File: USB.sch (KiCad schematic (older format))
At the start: 47 parts

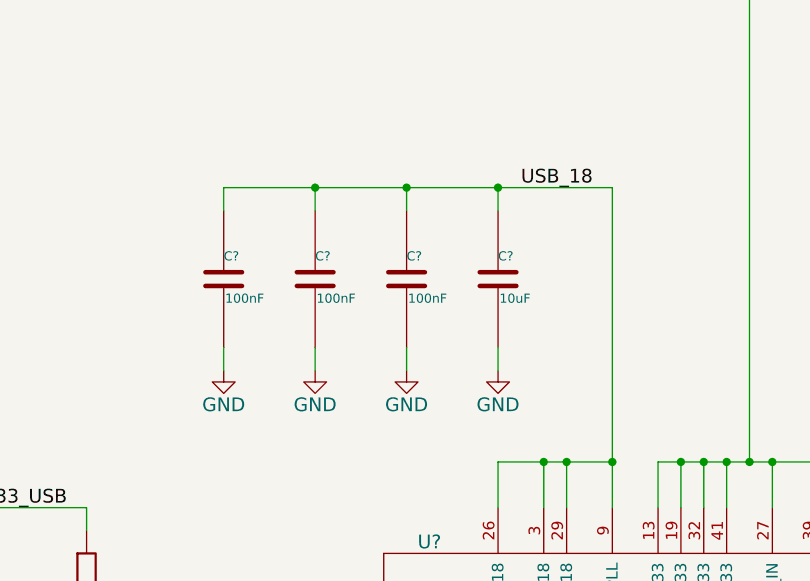
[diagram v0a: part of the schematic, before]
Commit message: moved a bunch of things around inside the schematics
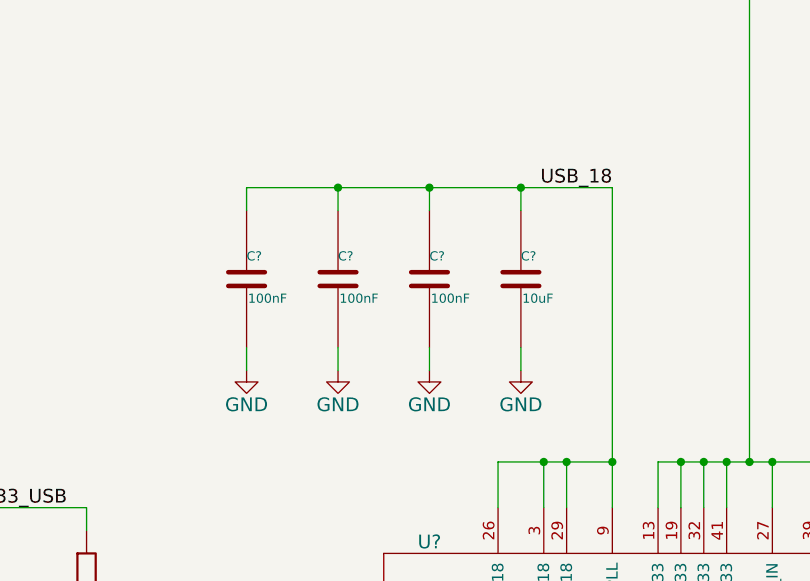
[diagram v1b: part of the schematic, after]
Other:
- moved on the sheet: C?
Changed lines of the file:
@@
 Text Label 13800 5900 0    60   ~ 0
 OVR#[2]
-Text Label 11400 3400 0    60   ~ 0
+Text Label 11800 3400 2    60   ~ 0
 USB_18
 $Comp
@@
 L TM_C C?
 U 1 1 54EDB9F5
-P 11300 3800
-F 0 "C?" H 11300 3900 40  0000 L CNN
-F 1 "10uF" H 11306 3715 40  0000 L CNN
-F 2 "tm-kicad-lib:SMD-0805-C" H 11338 3650 30  0001 C CNN
-F 3 "" H 11300 3800 60  0000 C CNN
-	1    11300 3800
+P 11400 3800
+F 0 "C?" H 11400 3900 40  0000 L CNN
+F 1 "10uF" H 11406 3715 40  0000 L CNN
+F 2 "tm-kicad-lib:SMD-0805-C" H 11438 3650 30  0001 C CNN
+F 3 "" H 11400 3800 60  0000 C CNN
+	1    11400 3800
 	1    0    0    -1
 $EndComp
@@
 L TM_C C?
 U 1 1 54EDB9FC
-P 10900 3800
-F 0 "C?" H 10900 3900 40  0000 L CNN
-F 1 "100nF" H 10906 3715 40  0000 L CNN
-F 2 "tm-kicad-lib:SMD-0402-C" H 10938 3650 30  0001 C CNN
-F 3 "" H 10900 3800 60  0000 C CNN
-	1    10900 3800
+P 11000 3800
+F 0 "C?" H 11000 3900 40  0000 L CNN
+F 1 "100nF" H 11006 3715 40  0000 L CNN
+F 2 "tm-kicad-lib:SMD-0402-C" H 11038 3650 30  0001 C CNN
+F 3 "" H 11000 3800 60  0000 C CNN
+	1    11000 3800
 	1    0    0    -1
 $EndComp
@@
 L TM_C C?
 U 1 1 54EDBA03
-P 10500 3800
-F 0 "C?" H 10500 3900 40  0000 L CNN
-F 1 "100nF" H 10506 3715 40  0000 L CNN
-F 2 "tm-kicad-lib:SMD-0402-C" H 10538 3650 30  0001 C CNN
-F 3 "" H 10500 3800 60  0000 C CNN
-	1    10500 3800
+P 10600 3800
+F 0 "C?" H 10600 3900 40  0000 L CNN
+F 1 "100nF" H 10606 3715 40  0000 L CNN
+F 2 "tm-kicad-lib:SMD-0402-C" H 10638 3650 30  0001 C CNN
+F 3 "" H 10600 3800 60  0000 C CNN
+	1    10600 3800
 	1    0    0    -1
 $EndComp
@@
 L TM_C C?
 U 1 1 54EDBA0A
-P 10100 3800
-F 0 "C?" H 10100 3900 40  0000 L CNN
-F 1 "100nF" H 10106 3715 40  0000 L CNN
-F 2 "tm-kicad-lib:SMD-0402-C" H 10138 3650 30  0001 C CNN
-F 3 "" H 10100 3800 60  0000 C CNN
-	1    10100 3800
+P 10200 3800
+F 0 "C?" H 10200 3900 40  0000 L CNN
+F 1 "100nF" H 10206 3715 40  0000 L CNN
+F 2 "tm-kicad-lib:SMD-0402-C" H 10238 3650 30  0001 C CNN
+F 3 "" H 10200 3800 60  0000 C CNN
+	1    10200 3800
 	1    0    0    -1
 $EndComp
@@
 L GND #PWR?
 U 1 1 54EB6EE4
-P 10100 4200
-F 0 "#PWR?" H 10100 3950 60  0001 C CNN
-F 1 "GND" H 10100 4050 60  0000 C CNN
-F 2 "" H 10100 4200 60  0000 C CNN
-F 3 "" H 10100 4200 60  0000 C CNN
-	1    10100 4200
+P 10200 4200
+F 0 "#PWR?" H 10200 3950 60  0001 C CNN
+F 1 "GND" H 10200 4050 60  0000 C CNN
+F 2 "" H 10200 4200 60  0000 C CNN
+F 3 "" H 10200 4200 60  0000 C CNN
+	1    10200 4200
 	1    0    0    -1
 $EndComp
@@
 L GND #PWR?
 U 1 1 54EB6F1C
-P 10500 4200
-F 0 "#PWR?" H 10500 3950 60  0001 C CNN
-F 1 "GND" H 10500 4050 60  0000 C CNN
-F 2 "" H 10500 4200 60  0000 C CNN
-F 3 "" H 10500 4200 60  0000 C CNN
-	1    10500 4200
+P 10600 4200
+F 0 "#PWR?" H 10600 3950 60  0001 C CNN
+F 1 "GND" H 10600 4050 60  0000 C CNN
+F 2 "" H 10600 4200 60  0000 C CNN
+F 3 "" H 10600 4200 60  0000 C CNN
+	1    10600 4200
 	1    0    0    -1
 $EndComp
@@
 L GND #PWR?
 U 1 1 54EB6F22
-P 10900 4200
-F 0 "#PWR?" H 10900 3950 60  0001 C CNN
-F 1 "GND" H 10900 4050 60  0000 C CNN
-F 2 "" H 10900 4200 60  0000 C CNN
-F 3 "" H 10900 4200 60  0000 C CNN
-	1    10900 4200
+P 11000 4200
+F 0 "#PWR?" H 11000 3950 60  0001 C CNN
+F 1 "GND" H 11000 4050 60  0000 C CNN
+F 2 "" H 11000 4200 60  0000 C CNN
+F 3 "" H 11000 4200 60  0000 C CNN
+	1    11000 4200
 	1    0    0    -1
 $EndComp
@@
 L GND #PWR?
 U 1 1 54EB6F5A
-P 11300 4200
-F 0 "#PWR?" H 11300 3950 60  0001 C CNN
-F 1 "GND" H 11300 4050 60  0000 C CNN
-F 2 "" H 11300 4200 60  0000 C CNN
-F 3 "" H 11300 4200 60  0000 C CNN
-	1    11300 4200
+P 11400 4200
+F 0 "#PWR?" H 11400 3950 60  0001 C CNN
+F 1 "GND" H 11400 4050 60  0000 C CNN
+F 2 "" H 11400 4200 60  0000 C CNN
+F 3 "" H 11400 4200 60  0000 C CNN
+	1    11400 4200
 	1    0    0    -1
 $EndComp
@@
 Connection ~ 12900 3400
 Wire Wire Line
-	10100 4200 10100 4100
-Wire Wire Line
-	10900 4200 10900 4100
-Wire Wire Line
-	10500 4200 10500 4100
-Wire Wire Line
-	11300 4200 11300 4100
-Wire Wire Line
-	10100 3400 10500 3400
-Wire Wire Line
-	10500 3400 10900 3400
-Wire Wire Line
-	10900 3400 11300 3400
-Wire Wire Line
-	11300 3400 11800 3400
-Wire Wire Line
-	11300 3400 11300 3500
-Wire Wire Line
-	10900 3500 10900 3400
-Connection ~ 10900 3400
-Wire Wire Line
-	10500 3500 10500 3400
-Connection ~ 10500 3400
-Wire Wire Line
-	10100 3500 10100 3400
-Connection ~ 11300 3400
+	10200 4200 10200 4100
+Wire Wire Line
+	11000 4200 11000 4100
+Wire Wire Line
+	10600 4200 10600 4100
+Wire Wire Line
+	11400 4200 11400 4100
+Wire Wire Line
+	10200 3400 10600 3400
+Wire Wire Line
+	10600 3400 11000 3400
+Wire Wire Line
+	11000 3400 11400 3400
+Wire Wire Line
+	11400 3400 11800 3400
+Wire Wire Line
+	11400 3400 11400 3500
+Wire Wire Line
+	11000 3500 11000 3400
+Connection ~ 11000 3400
+Wire Wire Line
+	10600 3500 10600 3400
+Connection ~ 10600 3400
+Wire Wire Line
+	10200 3500 10200 3400
+Connection ~ 11400 3400
 Wire Wire Line
 	13300 2700 13300 2600
